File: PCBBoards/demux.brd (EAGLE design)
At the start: 114.3 x 169.8 mm, 98 parts, among them IC1 4013N, IC2 4013N, IC3 4013N, IC4 4013N, IC5 4013N, IC6 4013N, IC7 4069N, IC8 4069N, Q1 2N3904, Q10 2N3904, Q11 2N3904, Q12 2N3904, Q2 2N3904, Q3 2N3904, Q4 2N3904, Q5 2N3904, Q6 2N3904, Q7 2N3904, Q8 2N3904, Q9 2N3904, T1 2N3904, T2 2N3904, T3 2N3904, T4 2N3904, T5 2N3904, T6 2N3904

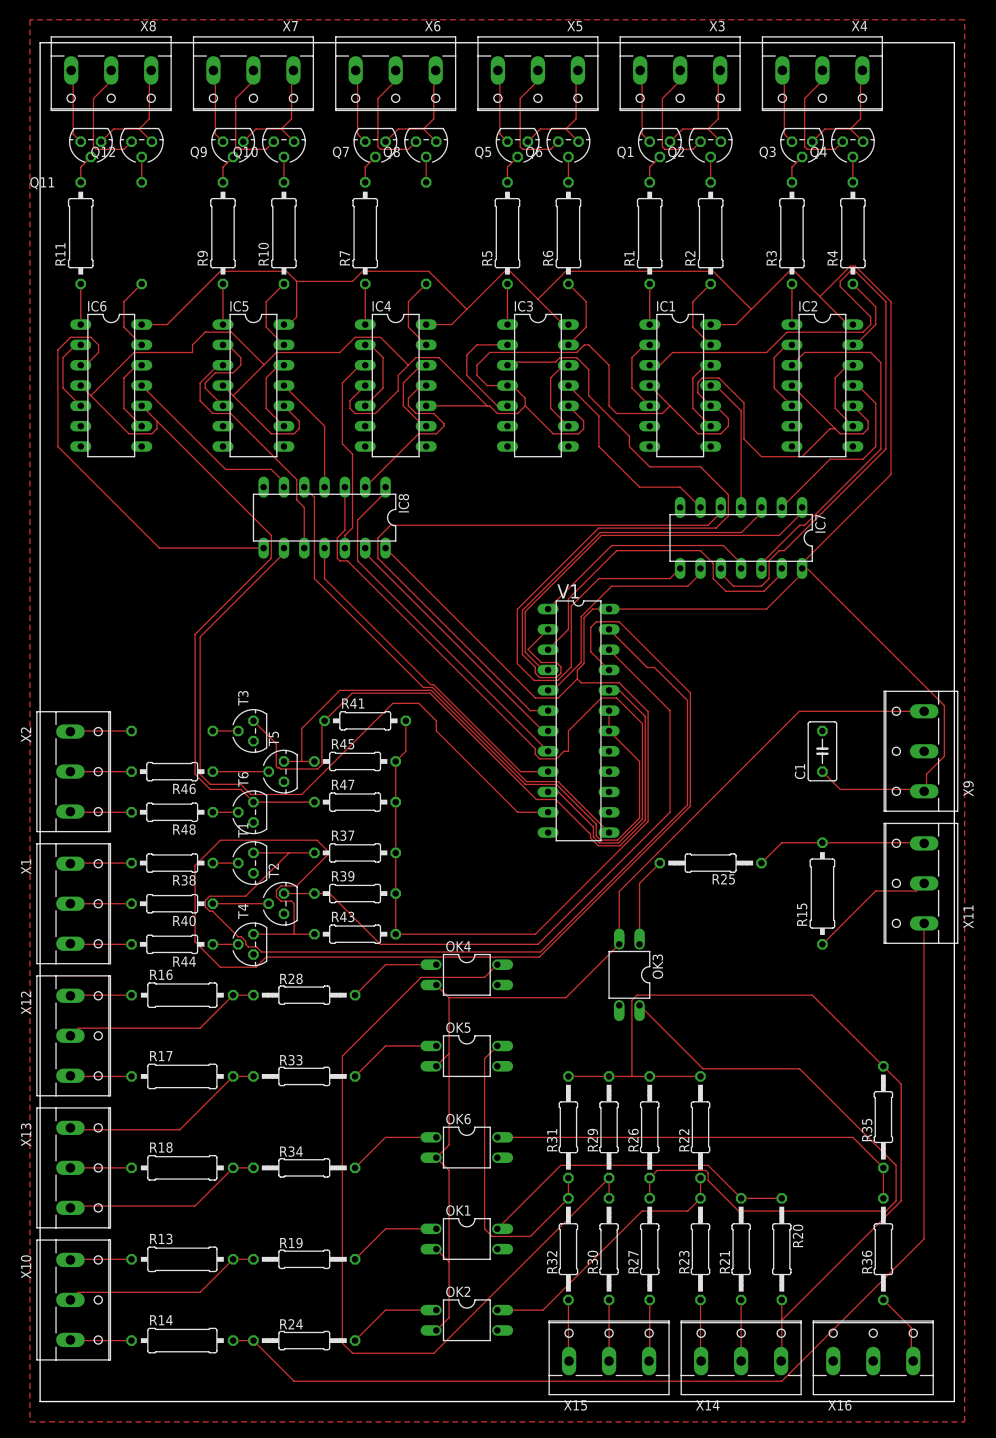
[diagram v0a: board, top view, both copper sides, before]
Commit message: FR/RS Board one of final update
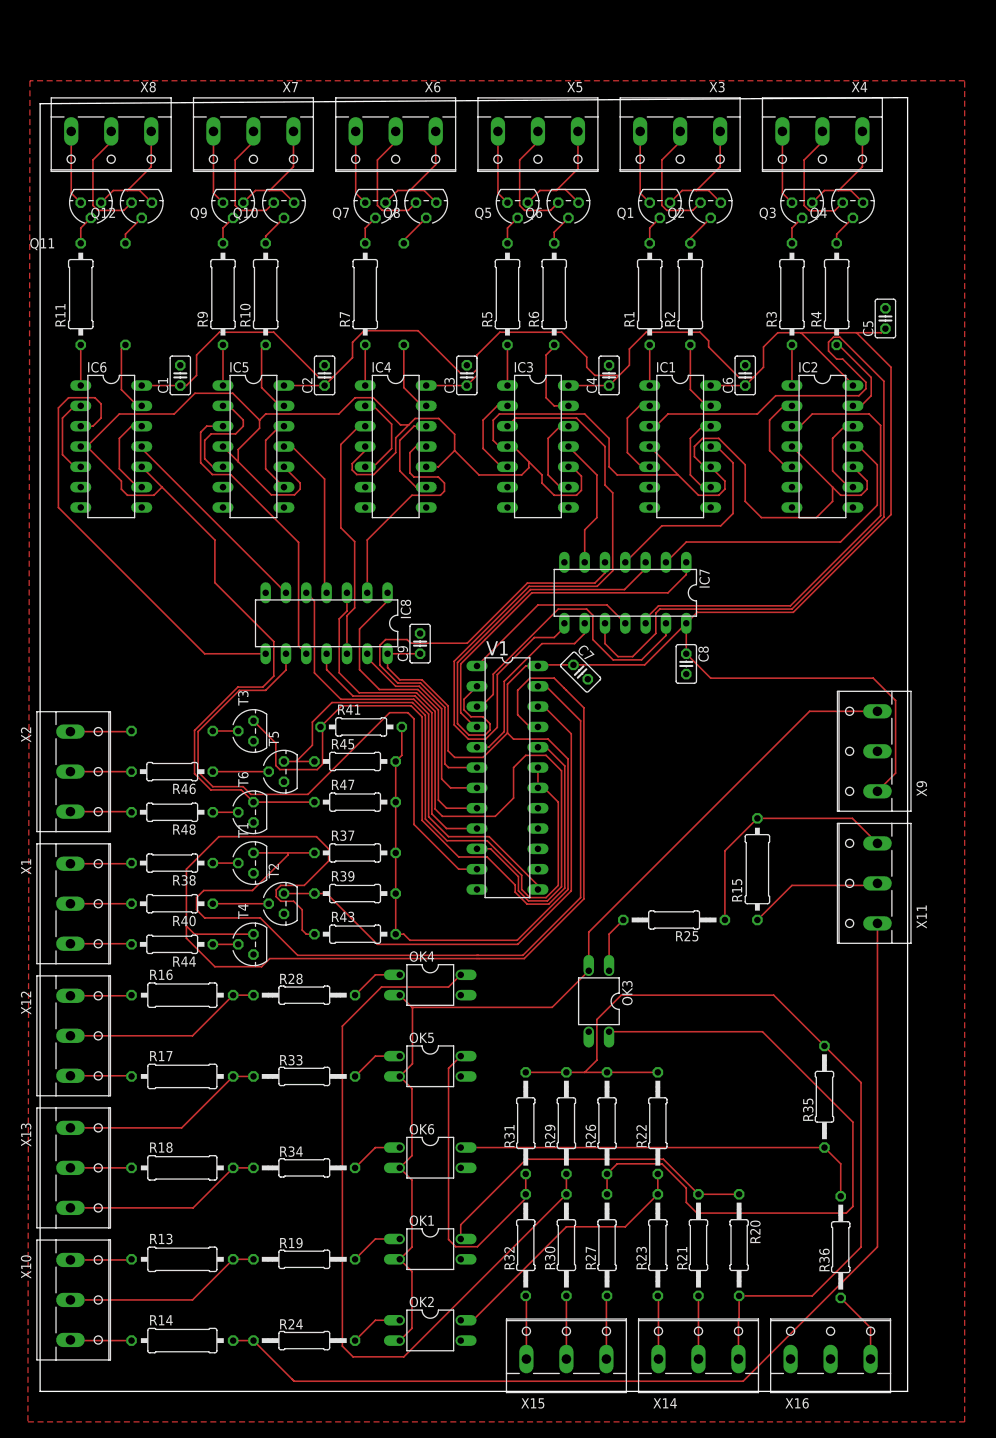
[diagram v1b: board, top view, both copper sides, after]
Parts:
- added C2, C3, C4, C5, C6, C7, C8, C9: 100n, rcl:C025-025X050
- C1: value 1u -> 100n; device rcl:C050-035X075 -> rcl:C025-025X050
- R19, R24, R25, R28, R33, R34: value 15k -> 4.7k
- moved C1 93.0 mm to (17.5, 58.4)
- moved IC7 16.0 mm to (73.2, 31.2)
- moved IC8 13.2 mm to (35.8, 27.4)
- moved V1 11.4 mm to (58.4, 8.13)
- moved R15 8.68 mm to (89.7, -3.30)
- moved R25 8.45 mm to (79.2, -9.65)
- moved R8 8.12 mm to (45.5, 68.6)
- moved R2 8.03 mm to (81.3, 68.6)
- moved R10 7.96 mm to (28.2, 68.6)
- moved R12 7.89 mm to (10.7, 68.6)
- moved R4 7.89 mm to (99.6, 68.6)
- moved R6 7.82 mm to (64.3, 68.6)
- moved R35 7.79 mm to (98.0, -31.8)
- moved R1 7.62 mm to (76.2, 68.6)
- moved R11 7.62 mm to (5.08, 68.6)
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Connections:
- net +5V: now also C2.1, C3.1, C4.1, C5.1, C6.1, C7.1, C8.1, C9.1
- net GND: now also C2.2, C3.2, C4.2, C5.2, C6.2, C7.2, C8.2, C9.2
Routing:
- net N$8: track 109.9 -> 87.1 mm
- net N$29: track 76.5 -> 57.7 mm
- net N$4: track 93.3 -> 110.4 mm
- net IN_1: track 81.2 -> 66.5 mm
- net N$1: track 44.6 -> 58.9 mm
- net N$2: track 24.1 -> 38.4 mm
- net IN_0: track 118.3 -> 105.6 mm
- net N$34: track 88.2 -> 77.3 mm
- net IN_5: track 312.4 -> 302.4 mm
- net FREQ3: track 21.5 -> 30.7 mm
- net N$3: track 17.2 -> 26.0 mm
- net N$66: track 105.5 -> 97.0 mm
- net IN_2: track 159.9 -> 151.4 mm
- net N$13: track 25.1 -> 16.6 mm
- net N$7: track 22.5 -> 29.5 mm
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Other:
- board size 114.3 x 169.8 mm -> 108.4 x 161.7 mm
